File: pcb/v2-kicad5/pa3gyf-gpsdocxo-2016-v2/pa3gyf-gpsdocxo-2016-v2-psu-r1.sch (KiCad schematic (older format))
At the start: 12 parts

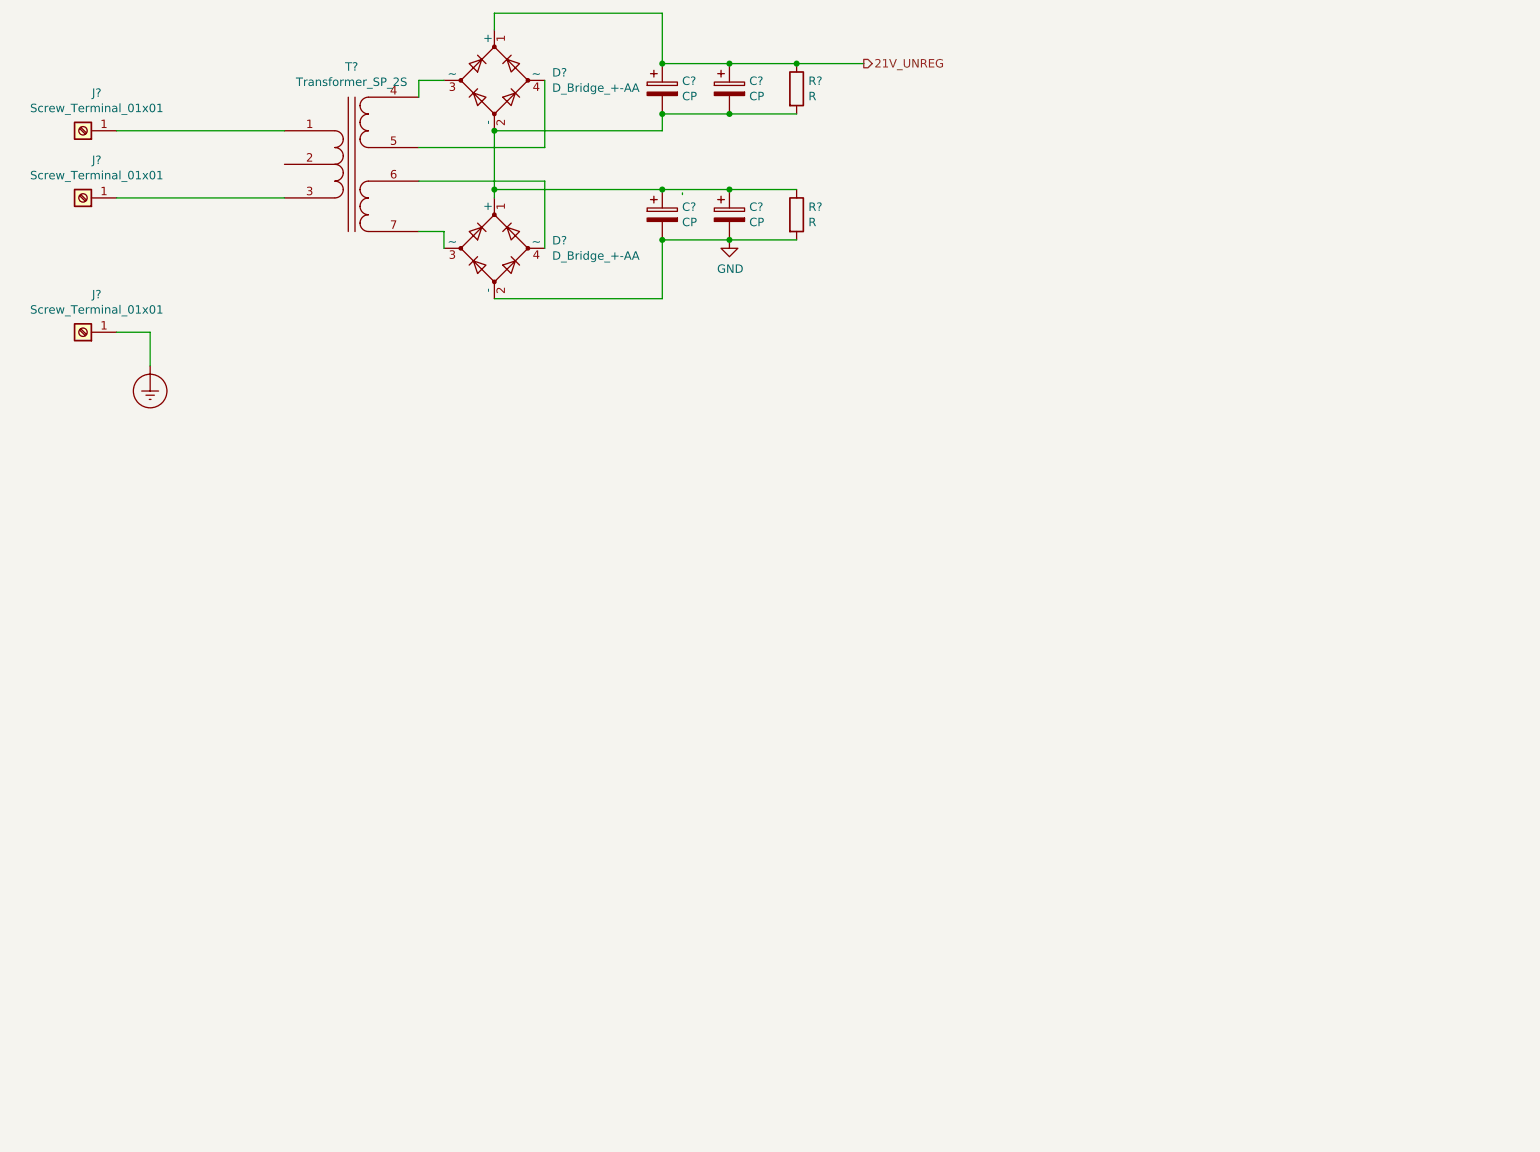
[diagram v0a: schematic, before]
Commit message: Committing apparent changes in working directory.
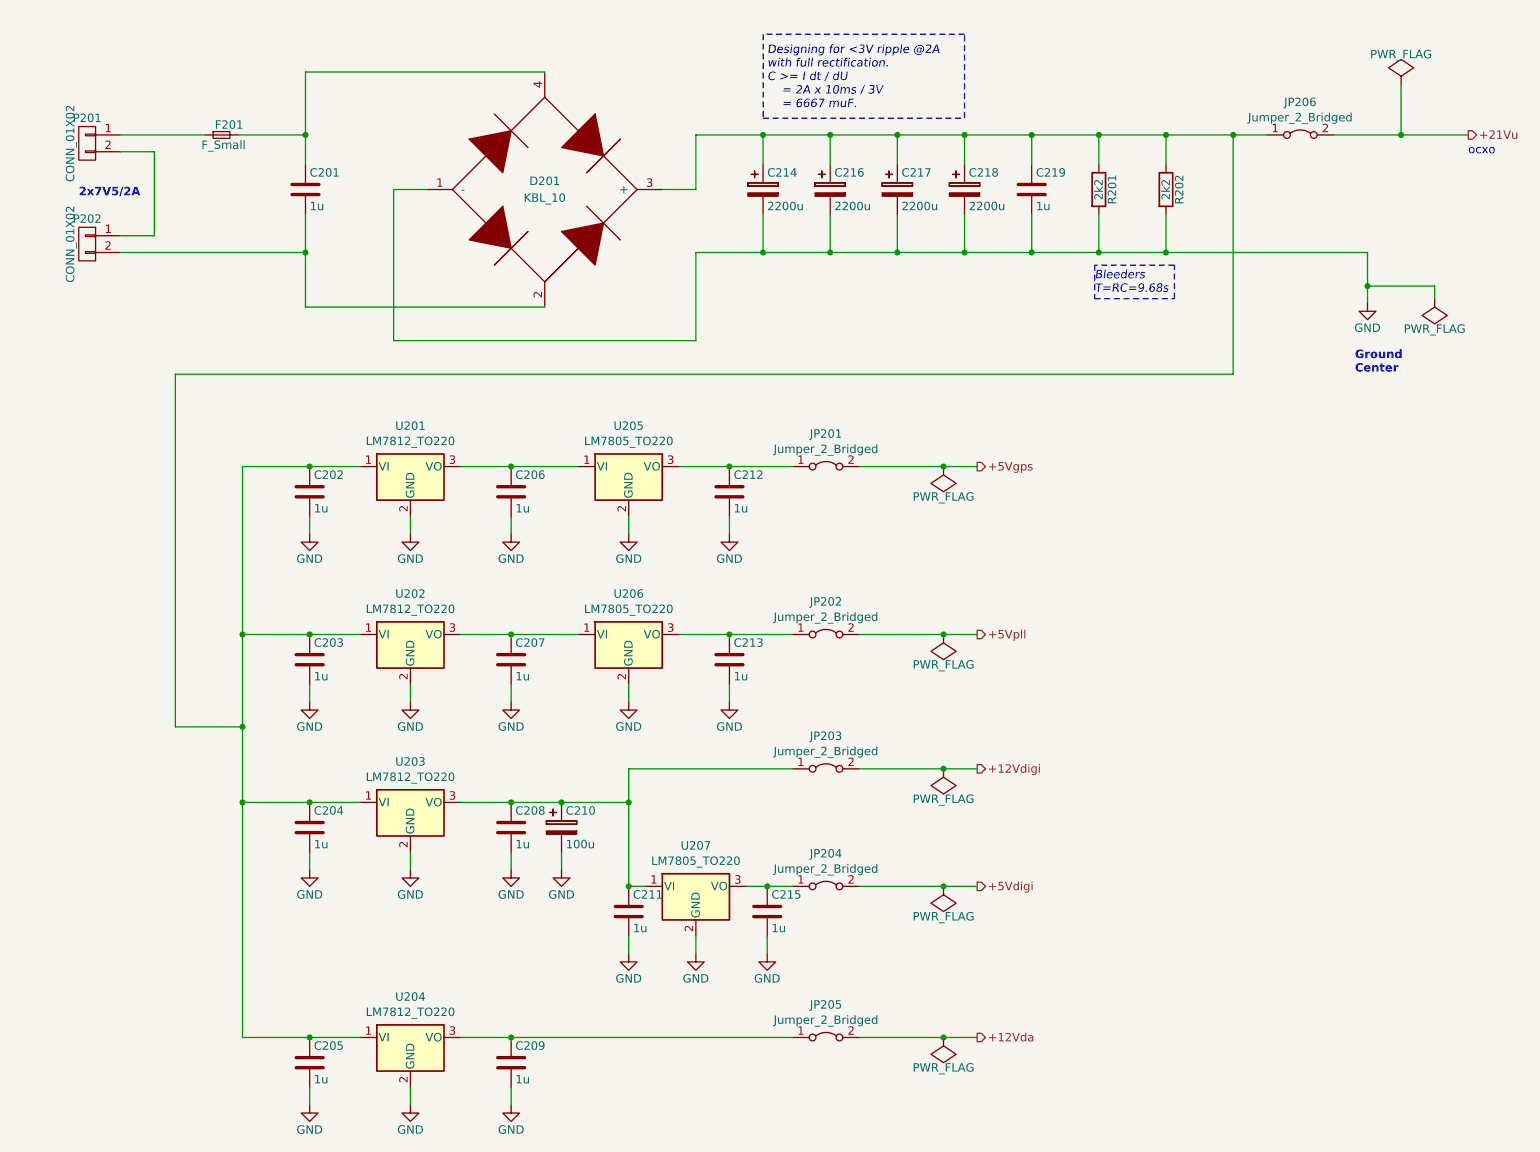
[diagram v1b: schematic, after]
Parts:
- removed C? (x4): CP, symbol Device:CP
- removed D? (x2): D_Bridge_+-AA, symbol Device:D_Bridge_+-AA
- removed J? (x3): Screw_Terminal_01x01, symbol Connector:Screw_Terminal_01x01
- removed R? (x2): R, symbol Device:R
- removed T?: Transformer_SP_2S, symbol Device:Transformer_SP_2S
- added C201, C202, C203, C204, C205, C206, C207, C208, C209, C211, C212, C213, C215, C219: 1u, Capacitors_SMD:C_0805_HandSoldering, symbol pa3gyf-gpsdocxo-2016-v2-rescue:C-pa3gyf-gpsdocxo-2016-psu-r3-cache-saved
- added C210: 100u, elkos:Elko_vert_30x16mm_RM7.5, symbol pa3gyf-gpsdocxo-2016-v2-rescue:CP-pa3gyf-gpsdocxo-2016-psu-r3-cache-saved
- added C214, C216, C217, C218: 2200u, elkos:Elko_vert_30x16mm_RM7.5, symbol pa3gyf-gpsdocxo-2016-v2-rescue:CP-pa3gyf-gpsdocxo-2016-psu-r3-cache-saved
- added D201: KBL_10, pa3gyf-kicad:Bridge_KBL, symbol pa3gyf-gpsdocxo-2016-v2-rescue:KBL_10-pa3gyf-gpsdocxo-2016-psu-r3-cache-saved
- added F201: F_Small, Fuse_Holders_and_Fuses:Fuseholder5x20_horiz_SemiClosed_Casing10x25mm, symbol pa3gyf-gpsdocxo-2016-v2-rescue:F_Small-pa3gyf-gpsdocxo-2016-psu-r3-cache-saved
- added JP201, JP202, JP203, JP204, JP205, JP206: Jumper_2_Bridged, symbol Jumper:Jumper_2_Bridged
- added P201, P202: CONN_01X02, weidmuller:Weidmuller_GS5_2_2pin, symbol pa3gyf-gpsdocxo-2016-v2-rescue:CONN_01X02-pa3gyf-gpsdocxo-2016-psu-r3-cache-sav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
- added R201, R202: 2k2, Resistors_ThroughHole:Resistor_Horizontal_RM15mm, symbol pa3gyf-gpsdocxo-2016-v2-rescue:R-pa3gyf-gpsdocxo-2016-psu-r3-cache-saved
- added U201, U202, U203, U204: LM7812_TO220, Package_TO_SOT_THT:TO-220-3_Vertical, symbol Regulator_Linear:LM7812_TO220
- added U205, U206, U207: LM7805_TO220, Package_TO_SOT_THT:TO-220-3_Vertical, symbol Regulator_Linear:LM7805_TO220
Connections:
- net labels added: +12Vda, +12Vdigi, +21Vu, +5Vdigi, +5Vgps, +5Vpll
- net labels removed: 21V_UNREG, Earth_Protective
- wire segments 32 -> 121
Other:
- note added: "2x7V5/2A"
- note added: "Bleeders\nT=RC=9.68s"
- note added: "Designing for <3V ripple @2A\nwith full rectification.\nC >= I dt / dU\n = 2A x 10ms / 3V\n = 6667 muF."
- note added: "Ground\nCenter"
- note added: "ocxo"
